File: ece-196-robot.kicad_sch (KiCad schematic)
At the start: 31 parts, among them J1 Screw_Terminal_01x02, J10 Conn_01x02_Socket, J4 Conn_01x02_Socket, J5 Conn_01x02_Socket, J6 Conn_01x04_Pin, J7 Conn_01x04_Pin, J8 Conn_01x20_Pin, J9 Conn_01x20_Pin, U1 L298N, U2 LM7805_TO220, U4 L298N

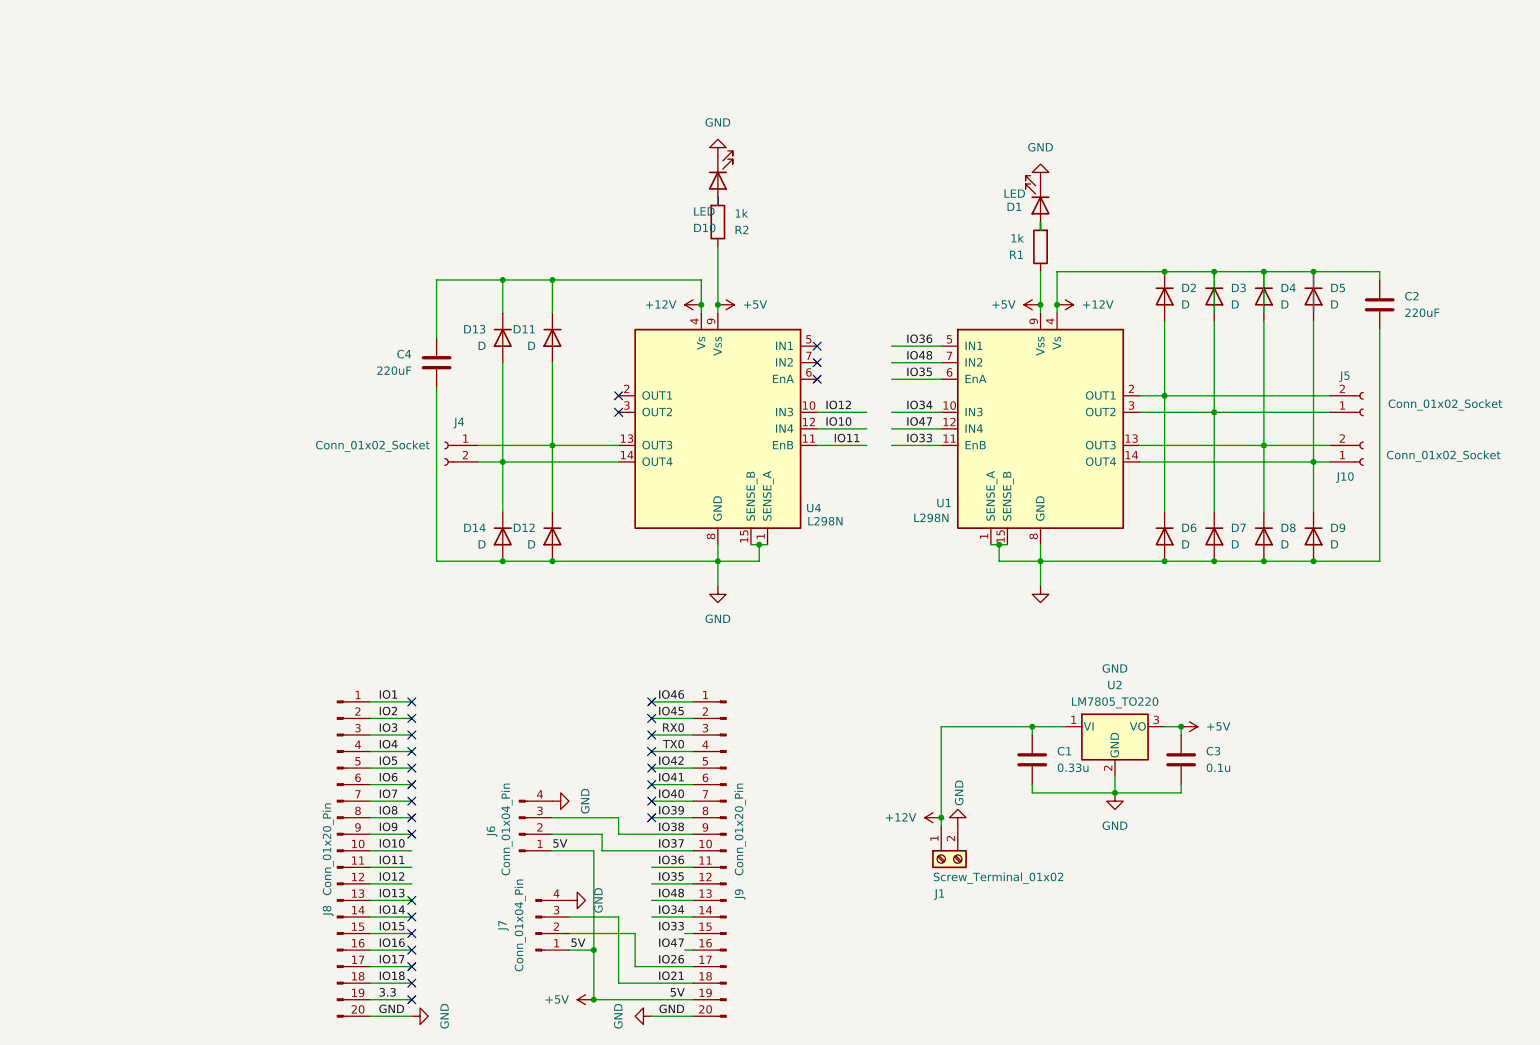
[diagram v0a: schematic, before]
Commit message: Update PCB schematic
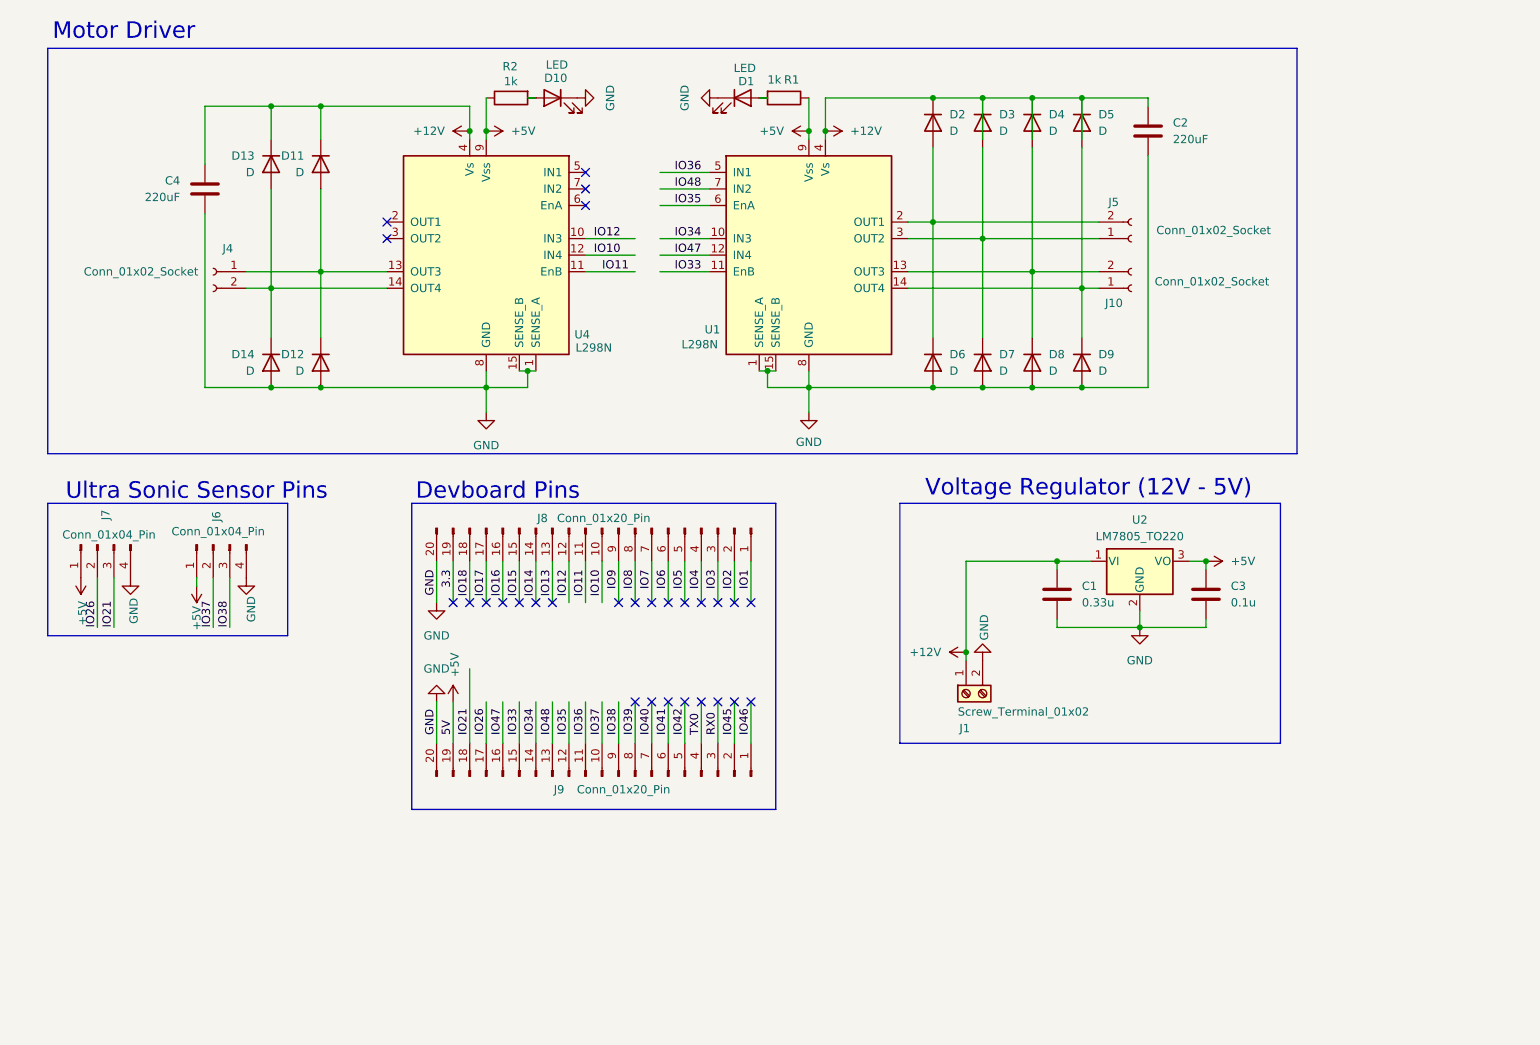
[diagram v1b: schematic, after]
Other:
- note added: "Devboard Pins"
- note added: "Motor Driver"
- note added: "Ultra Sonic Sensor Pins"
- note added: "Voltage Regulator (12V - 5V)"
- title: (none) -> ECE 196 FP PCB
- moved on the sheet: C1, C2, C3, C4, D1, D10, D11, D12, D13, D14, D2, D3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
